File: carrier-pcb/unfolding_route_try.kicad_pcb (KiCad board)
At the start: 2 copper layers, 66 parts, among them J1 USB_C_Receptacle_USB2.0, J2 Conn_01x04_Female, J3 1-338068-8, U1 TCA9548APWR, U10 DRV2605LDGS, U11 DRV2605LDGS, U12 BMX160, U2 TCA9548APWR, U3 DRV2605LDGS, U4 DRV2605LDGS, U5 DRV2605LDGS, U6 DRV2605LDGS, U7 DRV2605LDGS, U8 DRV2605LDGS, U9 DRV2605LDGS

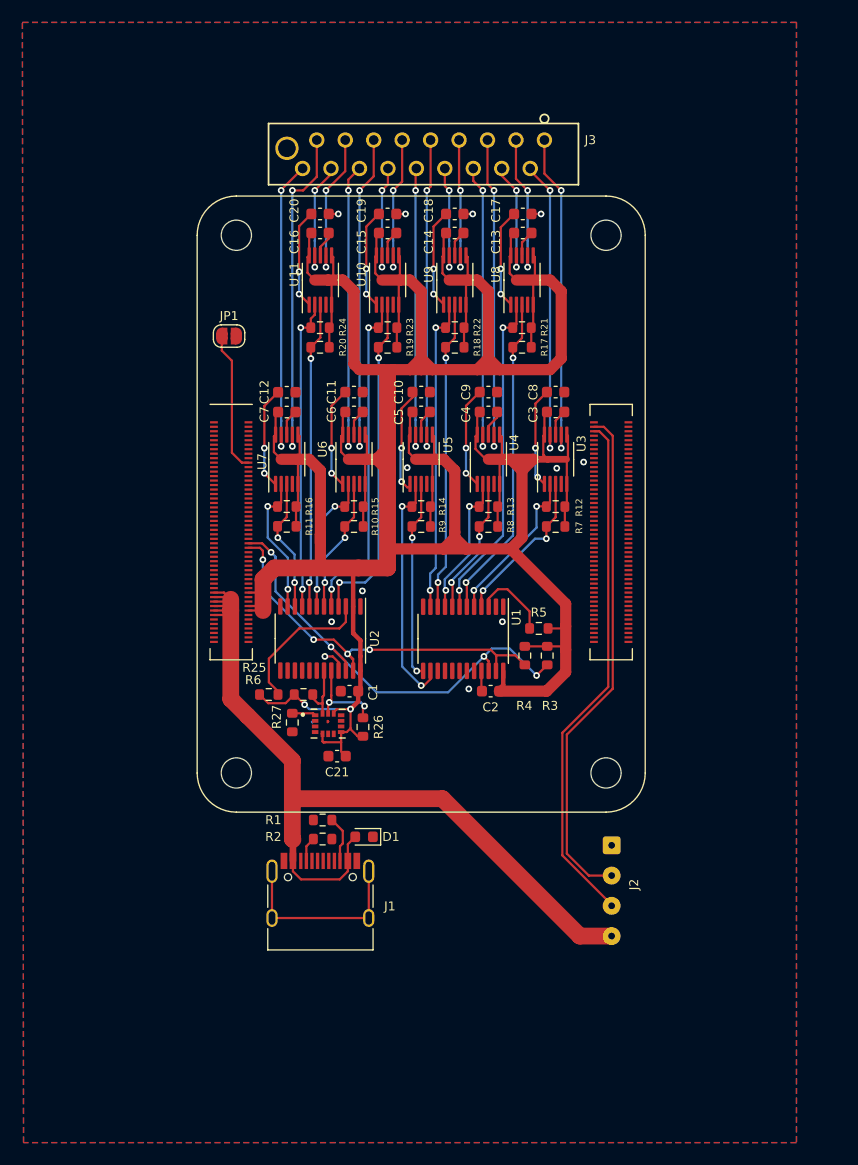
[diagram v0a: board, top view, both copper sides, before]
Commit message: New routing
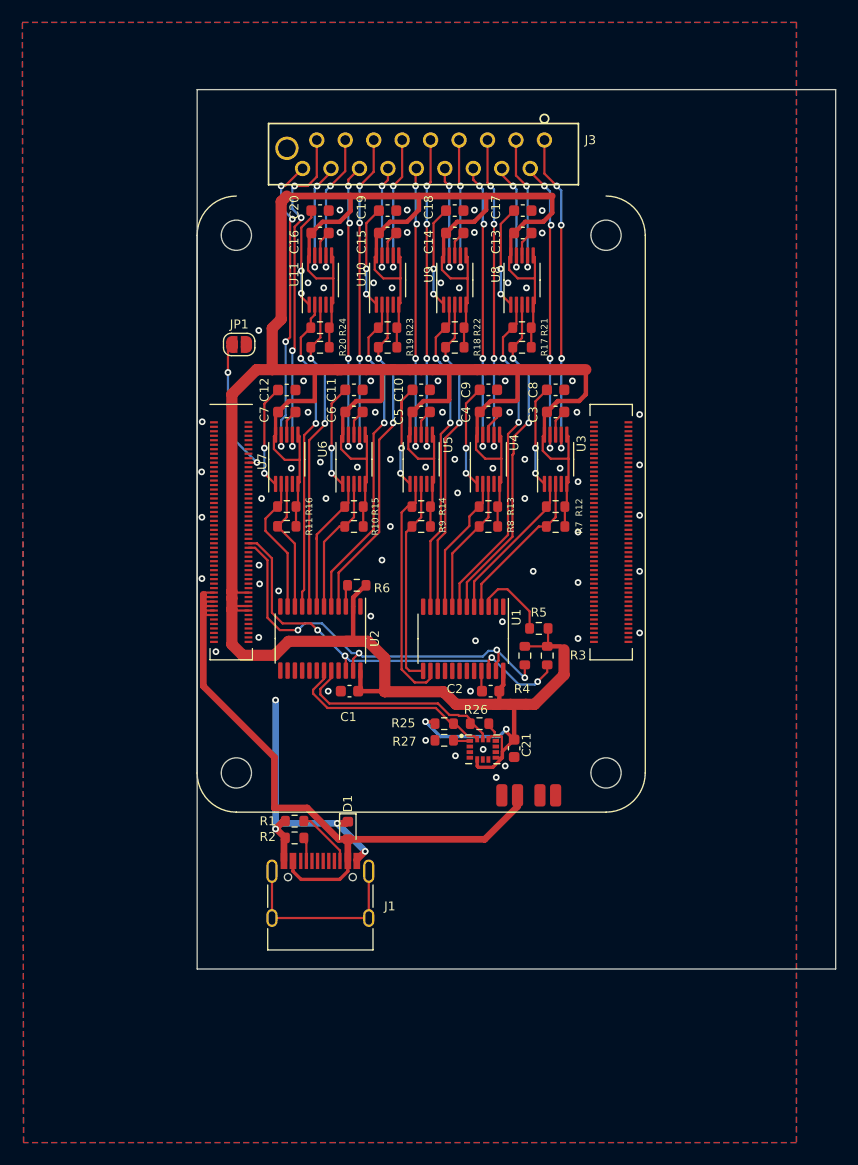
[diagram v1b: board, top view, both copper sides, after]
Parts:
- added J4: Conn_01x01_Female, Connector_Wire:SolderWirePad_1x01_SMD_1x2mm, F.Cu at (146.1, 89.0)
- added J5: Conn_01x01_Female, Connector_Wire:SolderWirePad_1x01_SMD_1x2mm, F.Cu at (147.5, 89.0)
- added J6: Conn_01x01_Female, Connector_Wire:SolderWirePad_1x01_SMD_1x2mm, F.Cu at (142.7, 89.0)
- J2: value Conn_01x04_Female -> Conn_01x01_Female; footprint Connector_Wire:SolderWire-0.1sqmm_1x04_P3.6mm_D0.4mm_OD1mm -> Connector_Wire:SolderWirePad_1x01_SMD_1x2mm
- moved C21 15.8 mm to (143.8, 84.8), turned to -90 degrees
- moved U12 14.0 mm to (141.0, 84.9)
- moved R27 13.7 mm to (137.6, 84.1), turned to 180 degrees
- moved R25 12.8 mm to (137.6, 82.6)
- moved R6 12.5 mm to (129.8, 70.2), turned to 180 degrees
- moved R26 10.4 mm to (140.7, 82.6), turned to 180 degrees
- moved J2 8.78 mm to (144.1, 89.0), turned to 180 degrees
- moved R2 2.50 mm to (124.2, 92.8), turned to 180 degrees
- moved R1 2.50 mm to (124.2, 91.3)
- moved D1 1.56 mm to (128.9, 92.1), turned to -90 degrees
- moved JP1 1.17 mm to (119.2, 48.8)
- moved C17 0.30 mm to (144.6, 36.8)
- moved C18 0.30 mm to (138.5, 36.8)
- moved C19 0.30 mm to (132.5, 36.8)
- moved C20 0.30 mm to (126.5, 36.8)
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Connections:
- J2 pad 1: GND -> +5V
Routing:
- net USB_D+: track 46.6 -> 0.00 mm
- net USB_D-: track 45.8 -> 0.00 mm
- net +3V3: track 342.2 -> 366.8 mm
- net GND: track 28.7 -> 49.8 mm, vias 12 -> 75
- net +5V: track 78.8 -> 62.1 mm
- net SDA_bmx160: track 5.28 -> 18.8 mm
- net Net-(R6-Pad2): track 13.2 -> 1.95 mm
- net SCL_bmx160: track 8.33 -> 19.2 mm, vias 2 -> 0
- net SCL7: track 18.1 -> 12.3 mm, vias 2 -> 0
- net SDA: track 35.1 -> 38.5 mm
- net SCL: track 41.2 -> 39.0 mm
- net SCL1: track 15.1 -> 13.8 mm, vias 2 -> 0
- net SDA2: track 29.1 -> 30.2 mm
- net Net-(J1-PadB5): track 4.16 -> 5.24 mm
- net SDA4: track 27.6 -> 28.6 mm
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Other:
- board outline added: 57 x 78.5 mm
